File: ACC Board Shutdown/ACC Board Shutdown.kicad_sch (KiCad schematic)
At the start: 33 parts, among them J1 IMD, J2 Shutdown IL, K1 DK1A1B-5V, K2 DK1A1B-5V, K3 DK1A1B-5V, K4 G6BK-1114P-US, U1 74AHC1G04, U1 HEF4093B, U1 LM555xN, U2 74AHC1GU04, U3 74AHC1GU04, U4 74AHC1GU04

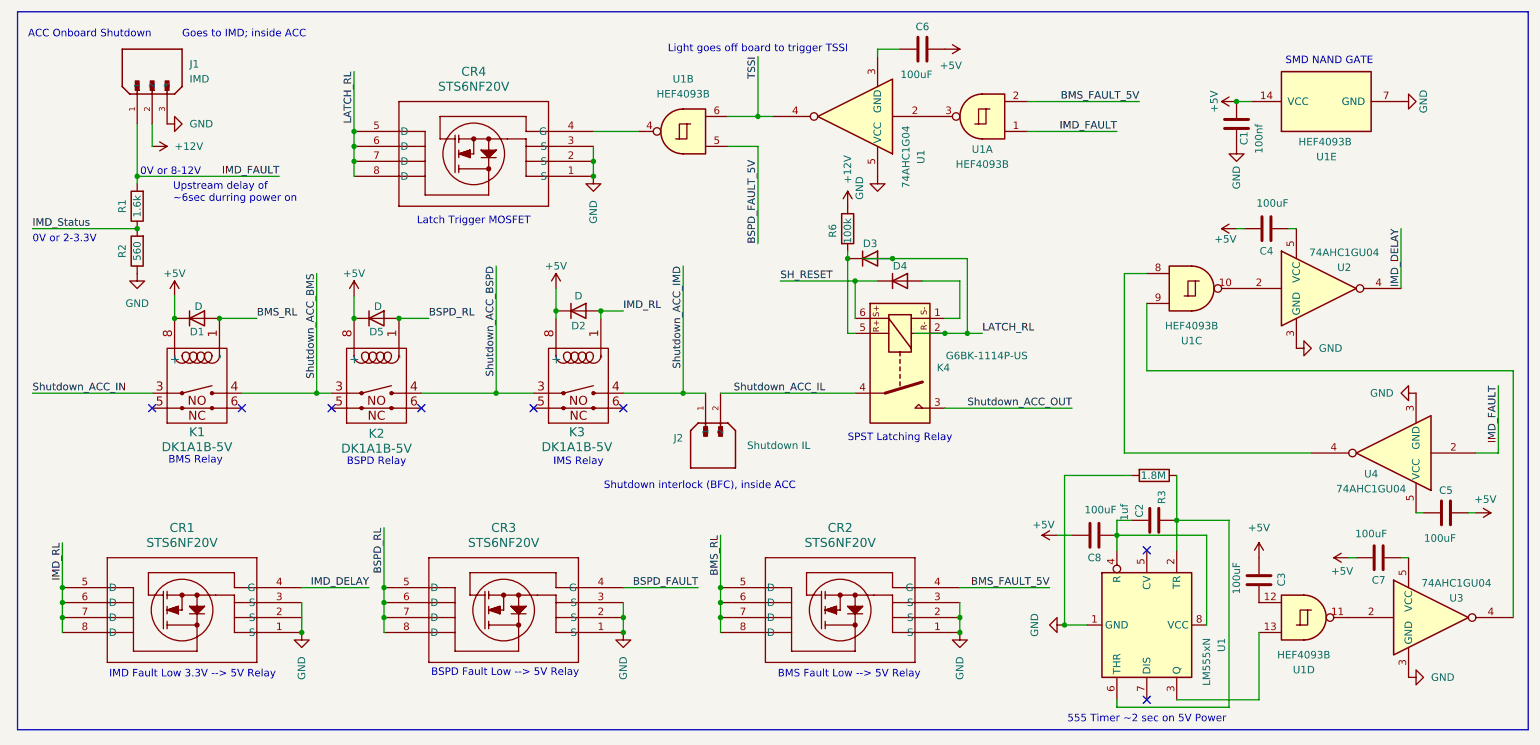
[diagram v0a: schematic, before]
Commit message: Update ACC Board Shutdown.kicad_sch
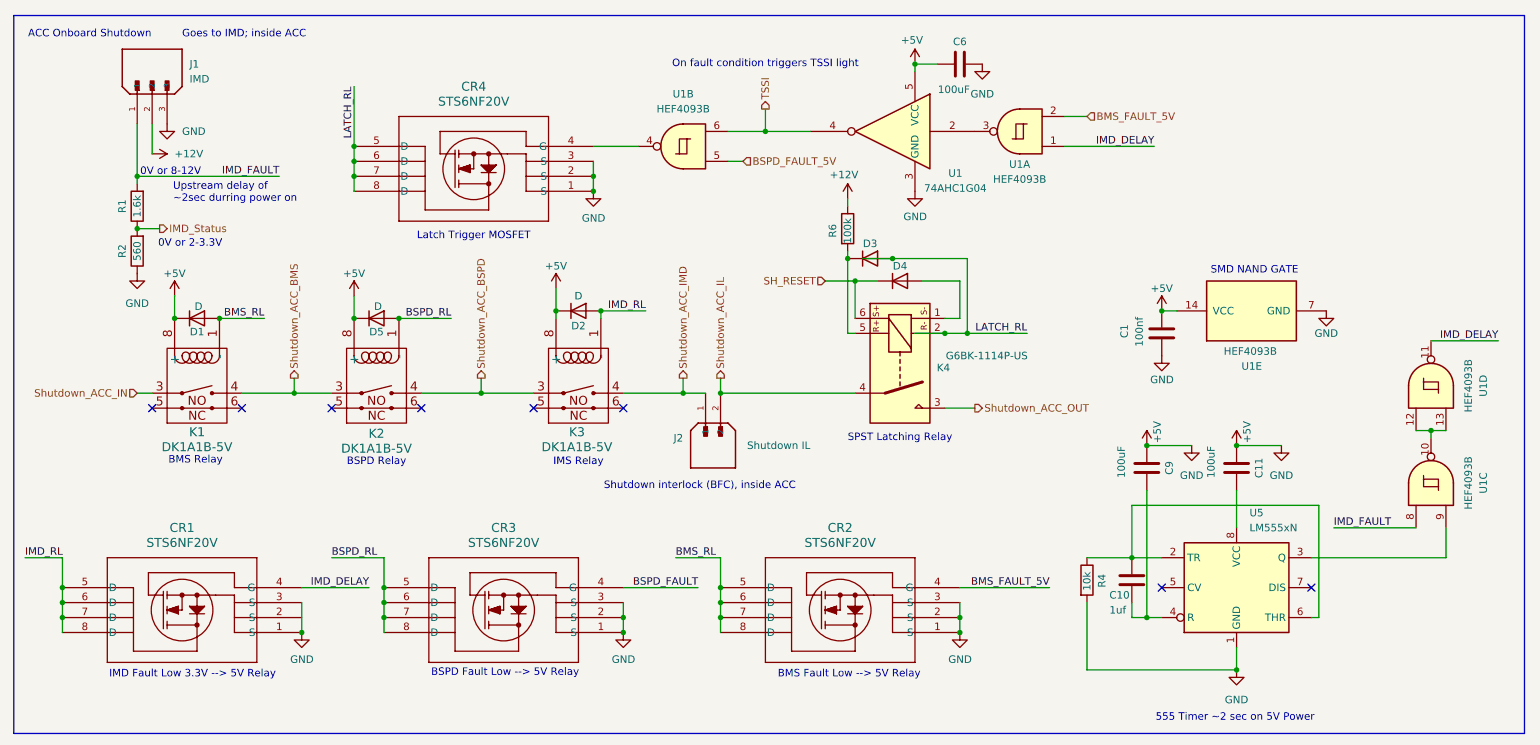
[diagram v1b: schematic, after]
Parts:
- removed C2: 1uf, symbol Device:C
- removed C3, C4, C5, C7, C8: 100uF, symbol Device:C
- removed R3: 1.8M, symbol Device:R
- removed U1: LM555xN, Package_DIP:DIP-8_W7.62mm, symbol Timer:LM555xN
- removed U2, U3, U4: 74AHC1GU04, symbol 74xGxx:74AHC1GU04
- added C10: 1uf, symbol Device:C
- added C11, C9: 100uF, symbol Device:C
- added R4: 10k, symbol Device:R
- added U5: LM555xN, Package_DIP:DIP-8_W7.62mm, symbol Timer:LM555xN
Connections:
- net GND is gone; now on net +5V: C1.1, CR1.1 (S), CR1.3 (S), CR2.1 (S), CR2.2 (S), CR2.3 (S), CR3.1 (S), CR3.2 (S), CR3.3 (S), CR4.1 (S), CR4.2 (S), CR4.3 (S), J1.3, R2.1, U1.5 (VCC), U1.7 (GND)
- net +5V: now also C6.1, U1.3 (GND), C11.1, C9.1, R4.2, U5.1 (GND)
- net IMD_DELAY: now also U1.1, U1.11
- net IMD_FAULT: now also U1.8; no longer U1.1
- net at U1.13: now also U1.10, U1.12
- net at U1.9: now also U5.3 (Q)
- new net: C10.2, C9.2, U5.4 (R)
- new net: C10.1, R4.1, U5.2 (TR), U5.6 (THR)
- new net: C11.2, U5.8 (VCC)
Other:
- note added: "On fault condition triggers TSSI light"
- note added: "Upstream delay of ~2sec durring power on"
- note removed: "Light goes off board to trigger TSSI"
- note removed: "Upstream delay of ~6sec durring power on"
- moved on the sheet: C1, C6, CR4, U1, U1A, U1B, U1E
